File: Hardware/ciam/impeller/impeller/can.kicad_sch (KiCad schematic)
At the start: 40 parts, among them J1 Micro-Fit_1x4P, SW1 SW_DIP_x06, U3 ISO1050DUB, U4 B0505MT-1WR4

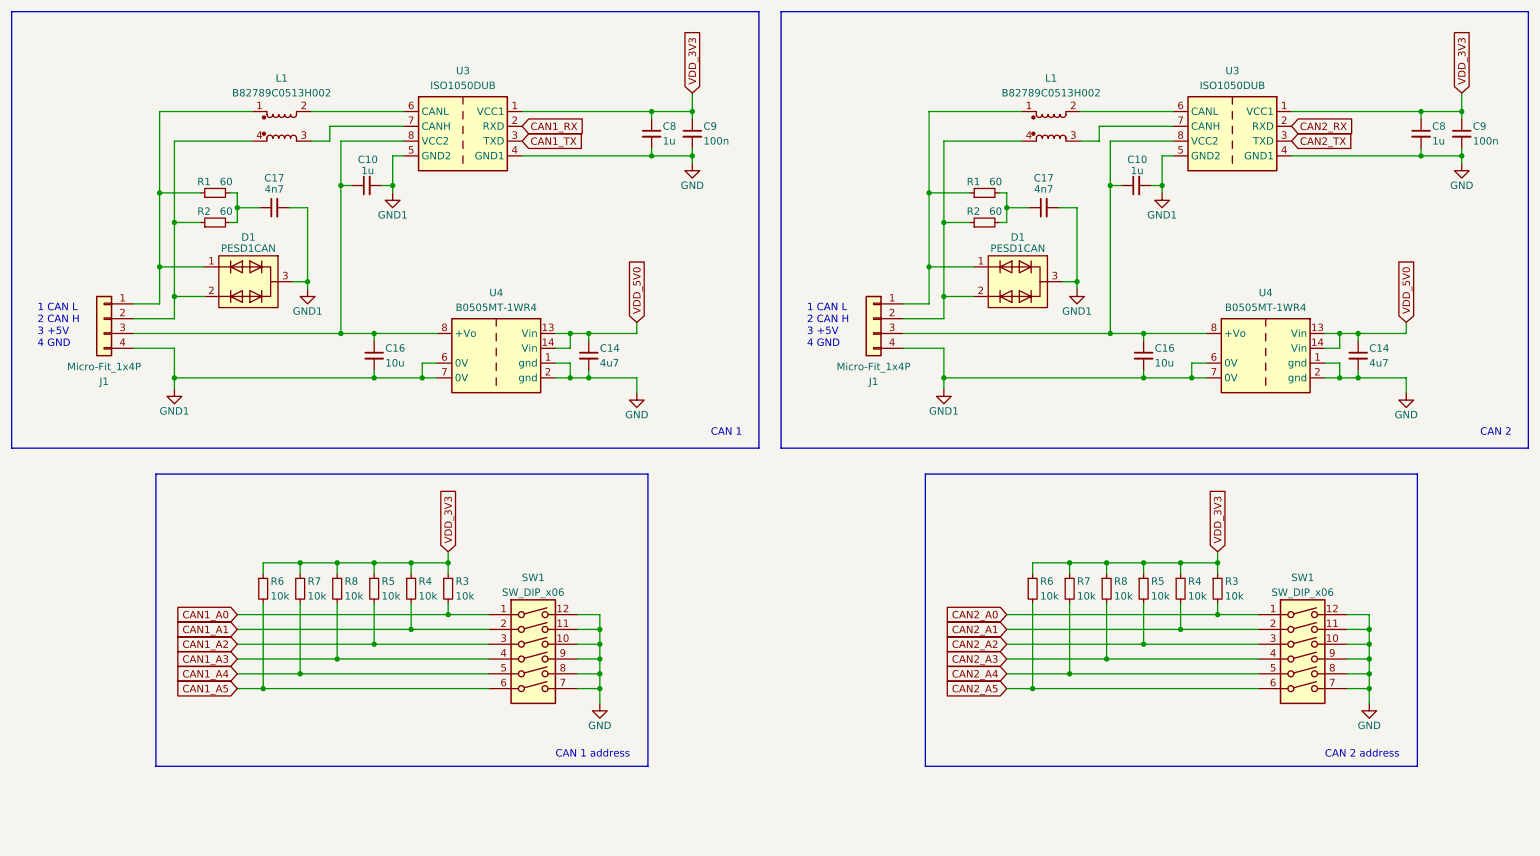
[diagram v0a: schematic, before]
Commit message: updated impeller project
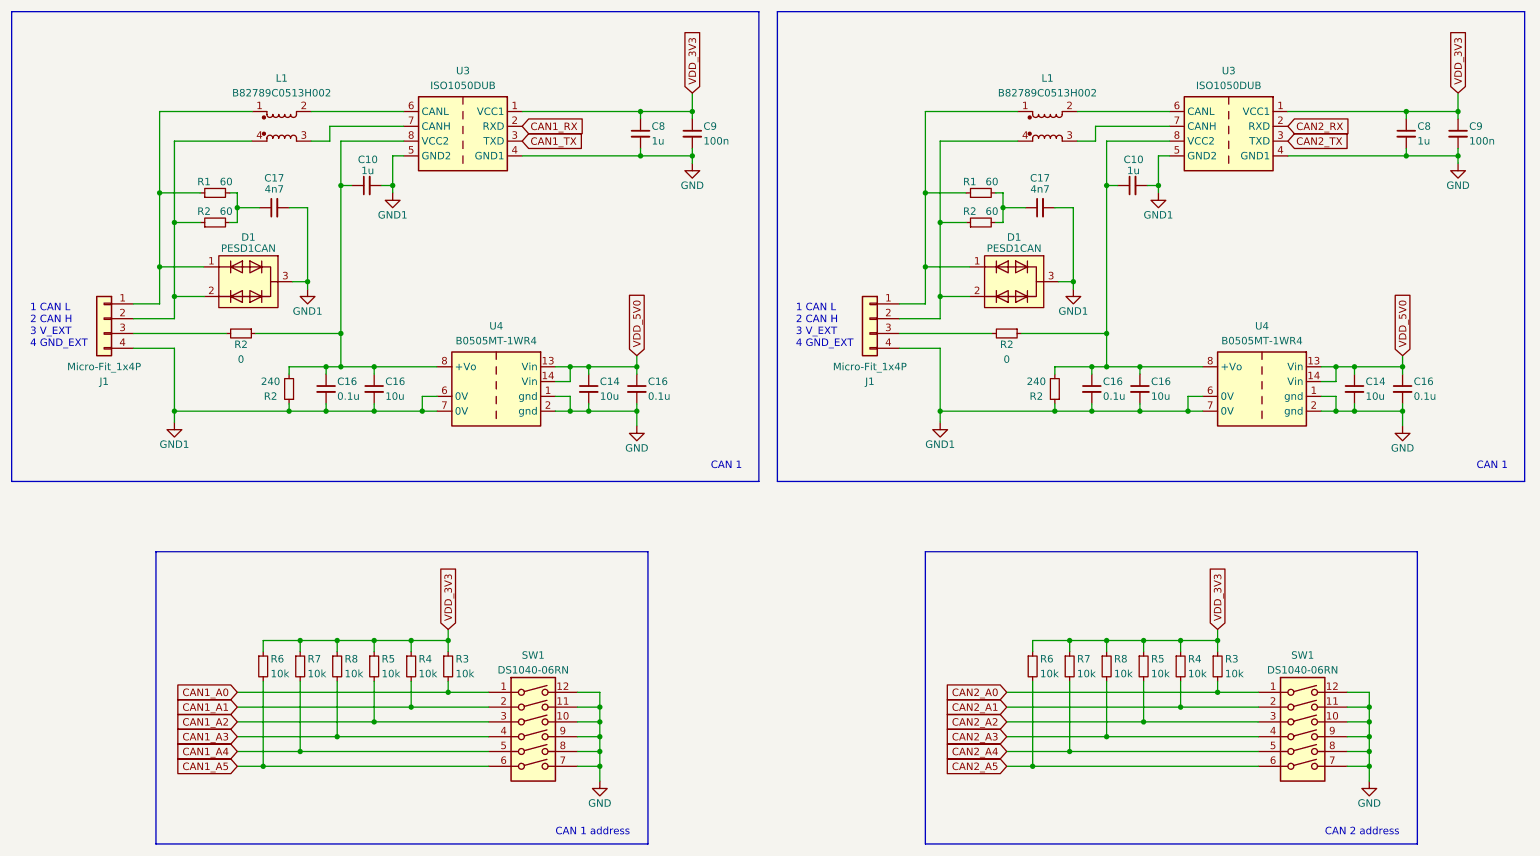
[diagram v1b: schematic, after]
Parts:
- removed C16: 10u, symbol Device:C_Small
- removed R2: 60, symbol Device:R_Small
- added C16: 10u, symbol Device:C_Small
- added C16 (x4): 0.1u, symbol Device:C_Small
- added R2 (x2): 240, symbol Device:R_Small
- added R2: 60, symbol Device:R_Small
- added R2 (x2): 0, symbol Device:R_Small
- C14: value 4u7 -> 10u
- SW1: value SW_DIP_x06 -> DS1040-06RN
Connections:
- net GND: now also C16.2, C16.2
- net GND1: now also C16.2, C16.2, C16.2, R2.1, R2.1
- net VDD_5V0: now also C16.1, C16.1
- net at D1.2, J1.2 (Pin_2), L1.4: now also R2.1
- net at C10.1, C16.1, U3.8 (VCC2)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: now also C16.1, R2.1, R2.2; no longer J1.3 (Pin_3)
- net at C17.1, R1.2: now also R2.2
- net at C10.1, U3.8 (VCC2), U4.8 (+Vo): now also C16.1, C16.1, R2.1, R2.2; no longer J1.3 (Pin_3)
- new net: J1.3 (Pin_3), R2.2 (x2)
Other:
- note added: "1 CAN L 2 CAN H 3 V_EXT 4 GND_EXT"
- note removed: "1 CAN L 2 CAN H 3 +5V 4 GND"
- note removed: "CAN 2"
- moved on the sheet: C14, C16, C8, R3, R4, R5, R6, R7, R8, SW1, U4
